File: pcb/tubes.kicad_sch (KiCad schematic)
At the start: 23 parts, among them Q10 MPSA42, Q11 MPSA42, Q12 MPSA42, Q13 MPSA42, Q4 MPSA42, Q5 MPSA42, Q6 MPSA42, Q7 MPSA42, Q8 MPSA42, Q9 MPSA42, U10 ISO7760DW

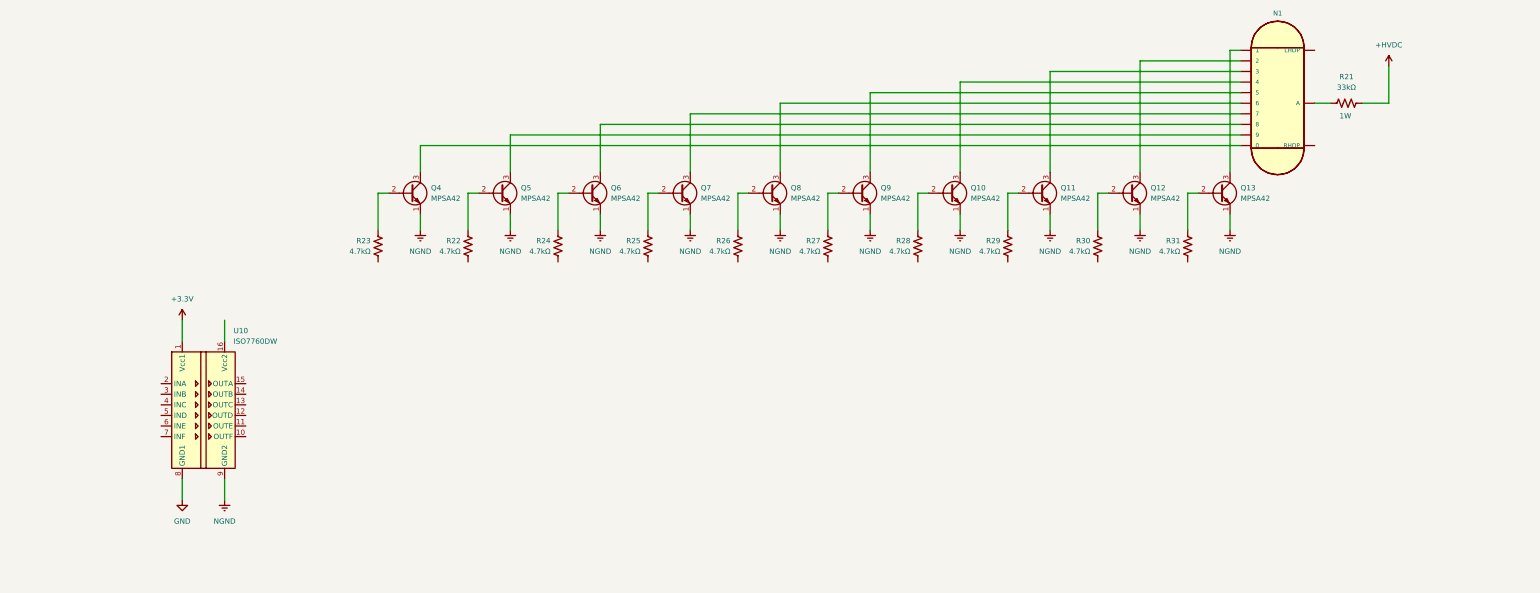
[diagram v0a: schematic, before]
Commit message: w
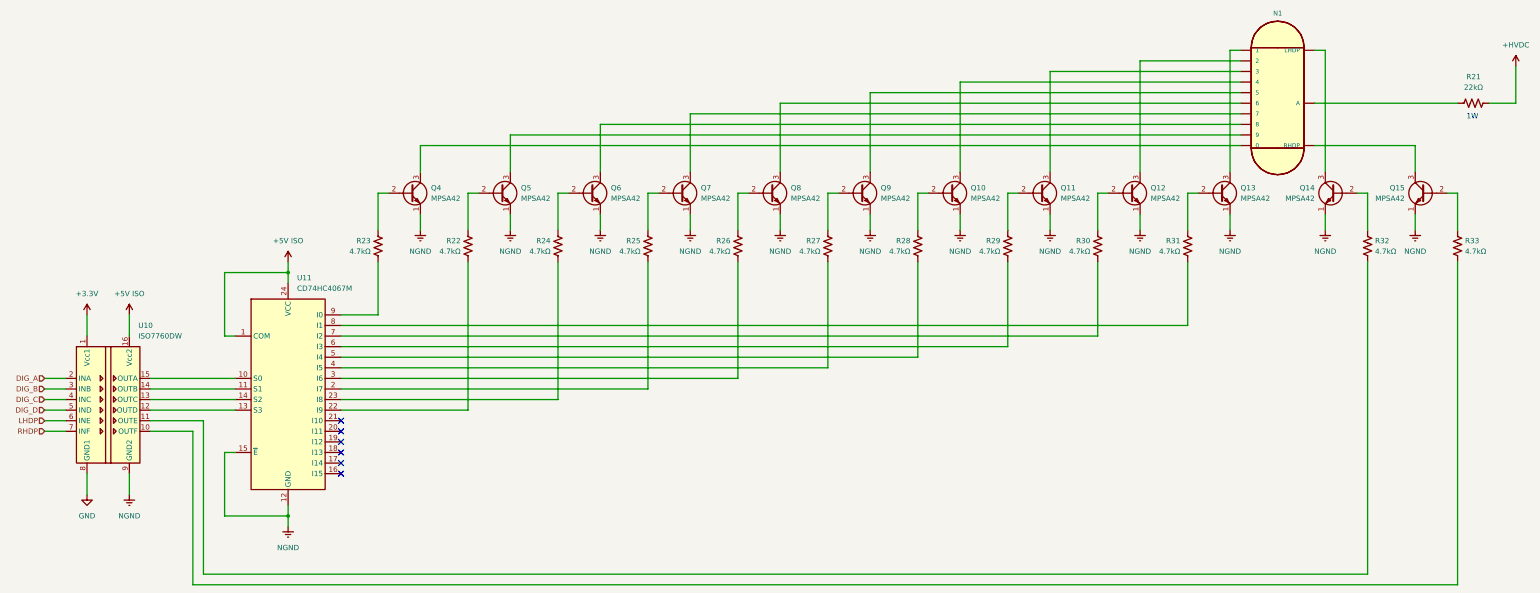
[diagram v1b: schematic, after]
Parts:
- added Q14, Q15: MPSA42, Package_TO_SOT_THT:TO-92_Inline, symbol Transistor_BJT:MPSA42
- added R32, R33: 4.7kΩ, Resistor_SMD:R_1206_3216Metric_Pad1.30x1.75mm_HandSolder, symbol Device:R_US
- added U11: CD74HC4067M, Package_SO:SOIC-24W_7.5x15.4mm_P1.27mm, symbol 74xx:CD74HC4067M
- R21: value 33kΩ -> 22kΩ
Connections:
- net NGND: now also Q14.1 (E), Q15.1 (E), U11.12 (GND), U11.15 (~{E})
- net at R22.1: now also U11.22 (I9)
- net at R29.1: now also U11.6 (I3)
- net at R28.1: now also U11.5 (I4)
- net at R23.1: now also U11.9 (I0)
- net at U10.10 (OUTF): now also R33.1
- net at U10.11 (OUTE): now also R32.1
- net at U10.12 (OUTD): now also U11.13 (S3)
- net at U10.13 (OUTC): now also U11.14 (S2)
- net at U10.14 (OUTB): now also U11.11 (S1)
- net at U10.15 (OUTA): now also U11.10 (S0)
- net +5V ISO: now reaches U10.16 (Vcc2)
- net +5V ISO: now also U11.1 (COM), U11.24 (VCC)
- net DIG_A: now reaches U10.2 (INA)
- net DIG_B: now reaches U10.3 (INB)
- net DIG_C: now reaches U10.4 (INC)
- net DIG_D: now reaches U10.5 (IND)
- net LHDP: now reaches U10.6 (INE)
- net RHDP: now reaches U10.7 (INF)
- net at R31.1: now also U11.8 (I1)
- net at R24.1: now also U11.23 (I8)
- net at R25.1: now also U11.2 (I7)
- net at R30.1: now also U11.7 (I2)
- net at N1.LHDP: now also Q14.3 (C)
- net at N1.RHDP: now also Q15.3 (C)
- net at R26.1: now also U11.3 (I6)
- net at R27.1: now also U11.4 (I5)
- new net: Q14.2 (B), R32.2
- new net: Q15.2 (B), R33.2
- no-connect marks 0 -> 6
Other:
- moved on the sheet: R21, U10
